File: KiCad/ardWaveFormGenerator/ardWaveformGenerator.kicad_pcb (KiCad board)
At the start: 2 copper layers, 108 x 52.7 mm, 24 parts, among them J1 Conn_Coaxial, J2 4-pin_I2C_LCD_header, U1 KY-040_Rotary_Encoder, U2 GY-9833_AD9833, U3 3-pole_Power_input_screw_term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, U4 TL071, U5 LM7812_TO220, U6 LM7912_TO220, U7 LM7805_TO220

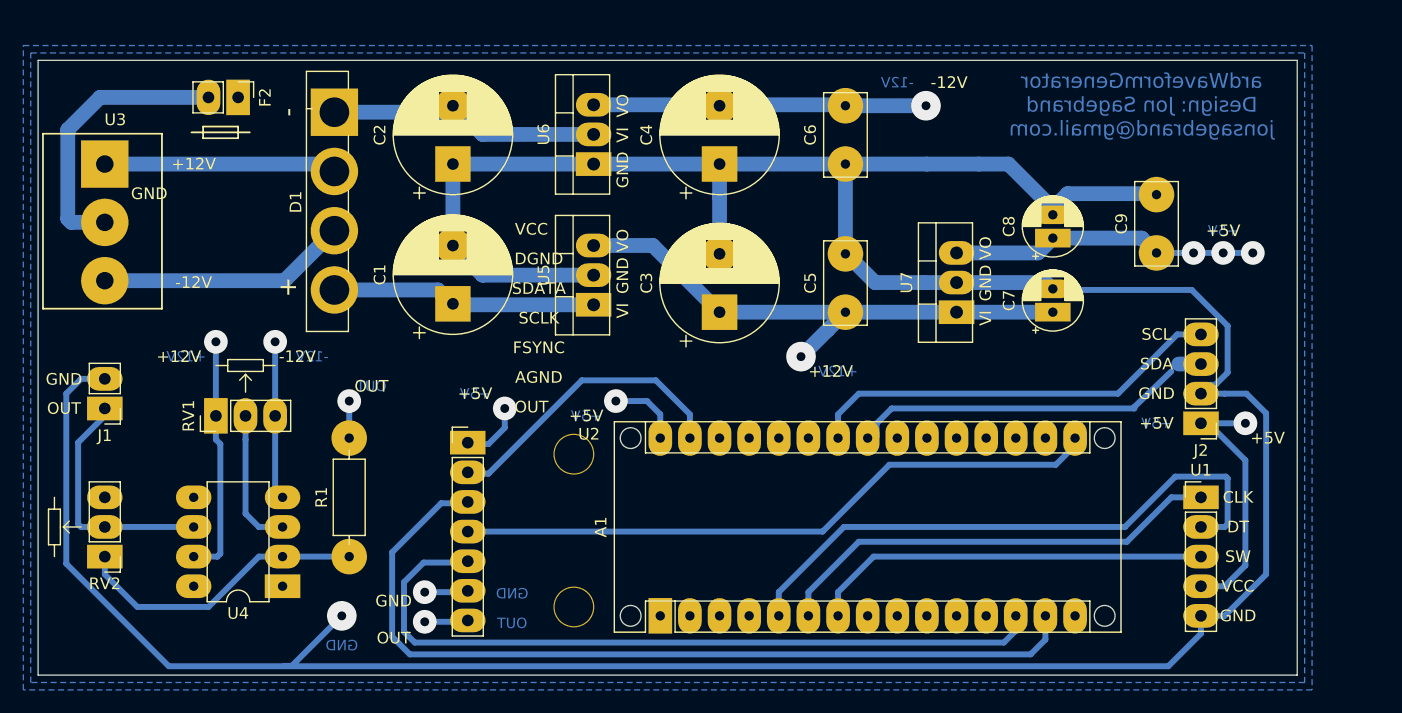
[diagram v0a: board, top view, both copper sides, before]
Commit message: ardWaveformGenerator-0.2
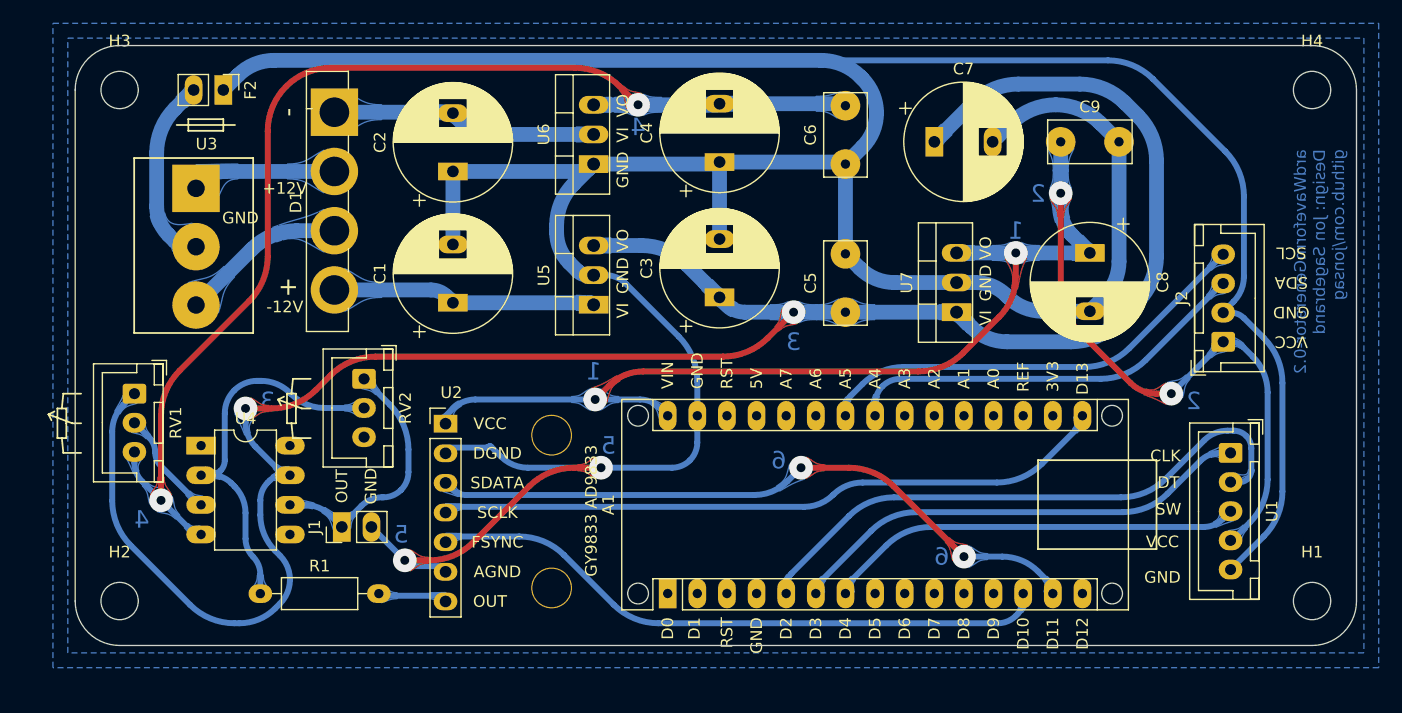
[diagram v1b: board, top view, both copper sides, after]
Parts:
- added H1: MountingHole, MountingHole:MountingHole_3.2mm_M3, F.Cu at (139.7, 108.0)
- added H2: MountingHole, MountingHole:MountingHole_3.2mm_M3, F.Cu at (37.5, 108.0)
- added H3: MountingHole, MountingHole:MountingHole_3.2mm_M3, F.Cu at (37.5, 64.1)
- added H4: MountingHole, MountingHole:MountingHole_3.2mm_M3, F.Cu at (139.7, 64.1)
- C7, C8: value 10u -> 1000u; footprint My_Misc:CP_Radial_D5.0mm_P2.00mm_larger -> My_Misc:CP_Radial_D10.0mm_P5.00mm_larger
- J2: footprint My_Headers:4-pin_I2C_LCD_header_larger -> My_Headers:4-pin JST LCD
- R1: footprint My_Misc:R_Axial_DIN0207_L6.3mm_D2.5mm_P10.16mm_Horizontal_larger_pads -> My_Misc:R_Axial_DIN0207_L6.3mm_D2.5mm_P10.16mm_Horizontal_large
- RV1, RV2: footprint My_Headers:3-pin_potentiometer_header_larger_pads -> My_Headers:3-pin JST Potentiometer
- U1: footprint My_Parts:3-pin_KY-040_Rotary_Encoder_header_large -> My_Headers:5-pin JST Rotary Encoder
- U2: footprint My_Parts:GY-9833_AD9833_larger -> My_Parts:GY-9833_AD9833_w_header_large
- moved RV2 26.9 mm to (58.4, 88.9), turned to -90 degrees
- moved J1 22.7 mm to (56.5, 101.6), turned to 90 degrees
- moved C7 17.8 mm to (107.3, 68.6), turned to 0 degrees
- moved U4 13.9 mm to (44.5, 94.6), turned to 0 degrees
- moved C9 12.6 mm to (118.2, 68.6), turned to 0 degrees
- moved R1 8.25 mm to (49.5, 107.3), turned to 0 degrees
- moved U3 8.09 mm to (44.0, 72.6)
- moved J2 7.24 mm to (132.1, 85.7), turned to 90 degrees
- moved RV1 7.24 mm to (38.7, 90.2), turned to -90 degrees
- moved U1 4.58 mm to (132.7, 95.2), turned to -90 degrees
- moved C8 3.42 mm to (120.7, 78.1), turned to -90 degrees
- moved A1 2.02 mm to (84.5, 107.3)
- moved U2 1.91 mm to (65.4, 92.7), turned to 0 degrees
- moved F2 1.42 mm to (46.4, 64.1)
- moved C3 1.27 mm to (88.9, 81.9)
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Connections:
- A1 pad 1: Net-(A1-Pad1) -> unconnected-(A1-Pad1)
- A1 pad 10: Net-(A1-Pad10) -> unconnected-(A1-Pad10)
- A1 pad 11: Net-(A1-Pad11) -> unconnected-(A1-Pad11)
- A1 pad 12: Net-(A1-Pad12) -> unconnected-(A1-Pad12)
- A1 pad 15: Net-(A1-Pad15) -> unconnected-(A1-Pad15)
- A1 pad 17: Net-(A1-Pad17) -> unconnected-(A1-Pad17)
- A1 pad 18: Net-(A1-Pad18) -> unconnected-(A1-Pad18)
- A1 pad 19: Net-(A1-Pad19) -> unconnected-(A1-Pad19)
- A1 pad 2: Net-(A1-Pad2) -> unconnected-(A1-Pad2)
- A1 pad 20: Net-(A1-Pad20) -> unconnected-(A1-Pad20)
- A1 pad 21: Net-(A1-Pad21) -> unconnected-(A1-Pad21)
- A1 pad 22: Net-(A1-Pad22) -> unconnected-(A1-Pad22)
- A1 pad 25: Net-(A1-Pad25) -> unconnected-(A1-Pad25)
- A1 pad 26: Net-(A1-Pad26) -> unconnected-(A1-Pad26)
- A1 pad 27: Net-(A1-Pad27) -> unconnected-(A1-Pad27)
- A1 pad 28: Net-(A1-Pad28) -> unconnected-(A1-Pad28)
- A1 pad 3: Net-(A1-Pad3) -> unconnected-(A1-Pad3)
- A1 pad 4: Net-(A1-Pad4) -> unconnected-(A1-Pad4)
- A1 pad 8: Net-(A1-Pad8) -> unconnected-(A1-Pad8)
- A1 pad 9: Net-(A1-Pad9) -> unconnected-(A1-Pad9)
- J2 pad 3: GND -> Net-(A1-Pad23)
- RV2 pad 1: Net-(R1-Pad1) -> Net-(J1-Pad1)
- RV2 pad 2: Net-(J1-Pad1) -> Net-(R1-Pad1)
- RV2 pad 3: Net-(RV2-Pad3) -> unconnected-(RV2-Pad3)
- U4 pad 1: Net-(U4-Pad1) -> unconnected-(U4-Pad1)
- U4 pad 5: Net-(U4-Pad5) -> unconnected-(U4-Pad5)
- U4 pad 8: Net-(U4-Pad8) -> unconnected-(U4-Pad8)
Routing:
- net +12V: track 67.8 -> 187.4 mm
- net +5V: track 60.3 -> 133.6 mm, vias 6 -> 4
- net -12V: track 42.1 -> 102.1 mm
- net Net-(A1-Pad14): track 74.4 -> 57.5 mm, vias 0 -> 2
- net Net-(A1-Pad13): track 63.4 -> 53.9 mm
- net Net-(D1-Pad3): track 21.5 -> 14.2 mm
- net Net-(F2-Pad2): track 23.5 -> 16.4 mm
- net Net-(R1-Pad1): track 25.4 -> 32.5 mm
- net Net-(D1-Pad2): track 19.0 -> 12.3 mm
- net GND: track 325.3 -> 330.9 mm
- net Net-(A1-Pad23): track 31.0 -> 35.2 mm
- net Net-(U4-Pad3): track 12.0 -> 9.30 mm
- net Net-(A1-Pad16): track 55.1 -> 57.7 mm
- net Net-(A1-Pad24): track 36.0 -> 38.3 mm
- net Net-(J1-Pad1): track 20.2 -> 22.3 mm
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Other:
- board size 108 x 52.7 mm -> 109.9 x 51.4 mm
- board text added: "${TITLE}-${REVISION} Design: Jon Sagebrand github.com/jonsag"
- board text added: "1"
- board text added: "2"
- board text added: "3"
- board text added: "4"
- board text added: "5"
- board text added: "6"
- board text removed: "+12V"
- board text removed: "+5V"
- board text removed: "-12V"
- board text removed: "GND"
- board text removed: "OUT"
- board text removed: "ardWaveformGenerator Design: Jon Sagebrand jonsagebrand@gmail.com"
